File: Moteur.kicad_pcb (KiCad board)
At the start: 4 copper layers, 28 x 16 mm, 56 parts, among them IC1 TPS71501, IC2 TLV710, IC3 MAX3051, IC4 LM5106, IC5 LM5106, IC6 INA282, P1 Bus2, P2 MotorEnc, P3 Bus1, P4 Motor, P5 DBG, P6 PWR, P7 GPIO, Q1 IRF8721, Q2 IRF8721, Q3 IRF8721, Q4 IRF8721, U1 STM32F303CCT6, X1 16MHz

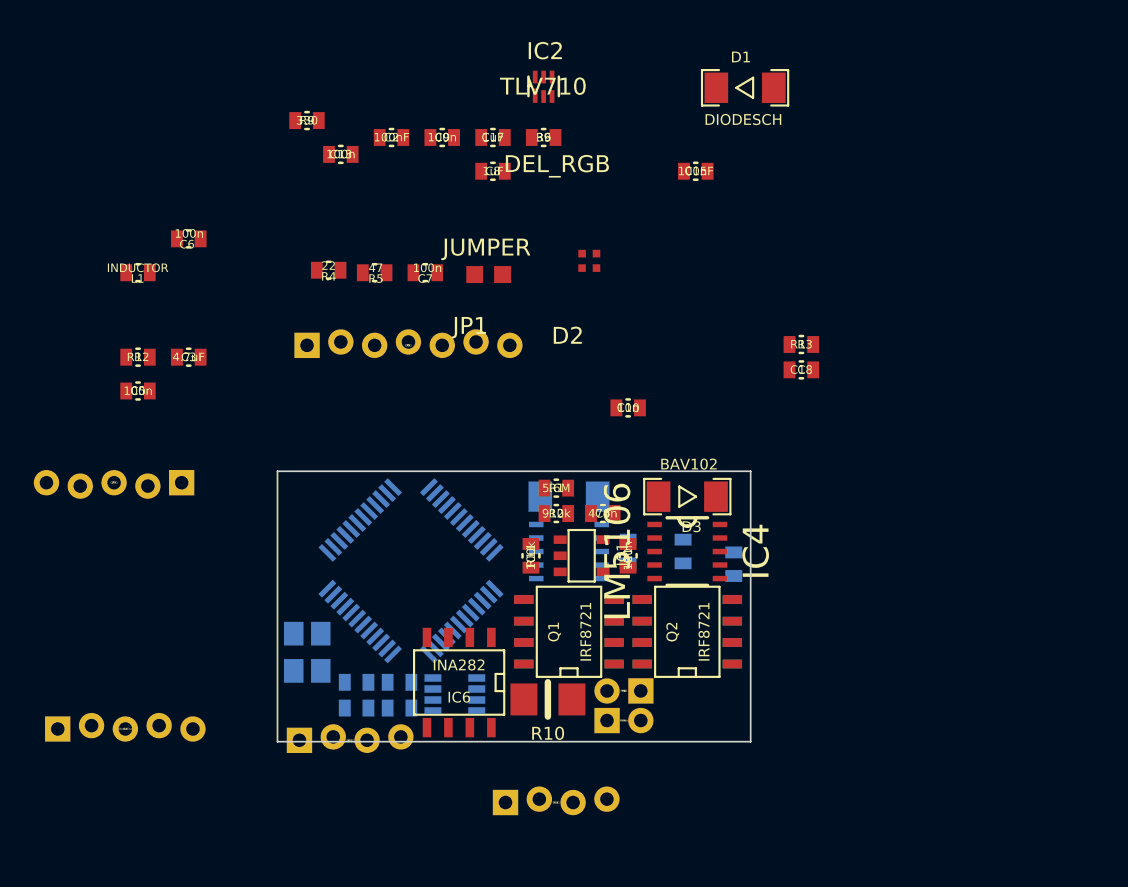
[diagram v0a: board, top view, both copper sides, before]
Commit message: final schematic review, component placement
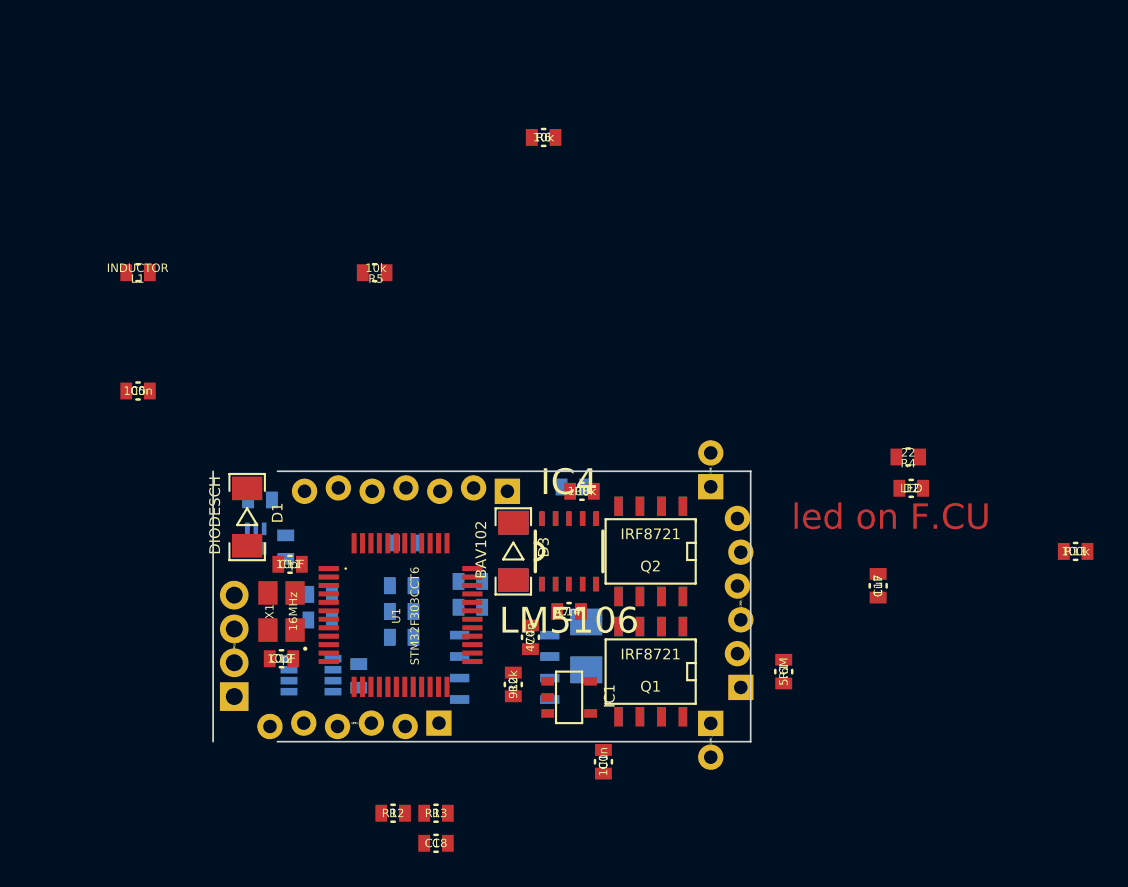
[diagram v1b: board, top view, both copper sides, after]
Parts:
- removed JP1: JUMPER, Jumer
- removed P7: GPIO, _Pin2mm_5z
- removed R7: 120, _0603
- C10, C13, C15, C2, C3, C6, C7, C8, C9, IC2, IC6, P5, R10, R9: moved to B.Cu
- C11, C12, C14, R8, U1, X1: moved to F.Cu
- D2: value DEL_RGB -> LED; footprint Led_RGB -> _0603
- P1: footprint _Pin2mm_4z -> pin4_can_connector
- P2: value MotorEnc -> CONN_6; footprint _Pin2mm_5z -> _Pin2mm_6z
- P3: value Bus1 -> GPIO; footprint _Pin2mm_4z -> _Pin2mm_6z
- P4: value Motor -> CONN_1
- P6: value PWR -> CONN_1
- R3: value 0R -> 10k
- R5: value 47 -> 10k
- R6: value 39 -> 10k
- moved D1 38.9 mm to (124.2, 92.7), turned to 270 degrees
- moved P2 37.2 mm to (153.4, 97.8), turned to 90 degrees
- moved R4 36.0 mm to (163.3, 89.2)
- moved C18 35.4 mm to (135.4, 112.0)
- moved R13 35.2 mm to (135.4, 110.2)
- moved C17 35.0 mm to (161.5, 96.8), turned to 270 degrees
- moved R11 32.2 mm to (173.2, 94.7), turned to 180 degrees
- moved IC2 31.7 mm to (124.7, 94.0)
- moved R12 30.9 mm to (132.8, 110.2)
- moved C13 30.9 mm to (130.8, 102.1), turned to 270 degrees
- moved R9 30.4 mm to (137.4, 98.0)
- moved C15 27.7 mm to (137.4, 96.5)
- moved C8 27.0 mm to (128.5, 97.3), turned to 180 degrees
- moved C9 26.6 mm to (133.3, 96.8)
- moved C6 25.4 mm to (133.3, 98.3)
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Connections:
- C15 pad 1: ADC/I_BAT -> ADC/I_MOT
- C5 pad 1: N-0000022 -> Reset
- IC3 pad 8: N-0000013 -> CAN_SPEED
- P2 pad 1: I -> Mot-
- P2 pad 2: B -> Mot+
- P2 pad 3: A -> GND
- P2 pad 4: GND -> +5V_protected
- P2 pad 5: +5V_protected -> B
- P3 pad 1: CANL -> GPIO_ADC
- P3 pad 2: CANH -> I
- P3 pad 3: GND -> GPIO_B
- P3 pad 4: +5V -> GPIO_A
- P4 pad 1: Mot- -> +BATT
- P4 pad 2: Mot+ -> (no net)
- P5 pad 3: (no net) -> Swdclk
- P5 pad 4: (no net) -> Swdio
- P5 pad 5: (no net) -> Reset
- P6 pad 2: +BATT -> (no net)
- R3 pad 1: N-0000012 -> +5V_protected
- R3 pad 2: N-0000013 -> GPIO_A
- R4 pad 1: N-0000068 -> LED
- R5 pad 1: N-0000069 -> +5V_protected
- R5 pad 2: N-0000067 -> GPIO_B
- R6 pad 1: LEDR -> +5V_protected
- R6 pad 2: N-0000046 -> I
- R9 pad 1: ADC/I_BAT -> ADC/I_MOT
- U1 pad 10: (no net) -> GPIO_ADC
- U1 pad 11: (no net) -> LED
- U1 pad 12: LEDR -> (no net)
- U1 pad 13: N-0000068 -> (no net)
- U1 pad 14: ADC/V_BAT -> CAN_SPEED
- U1 pad 15: (no net) -> ADC/I_MOT
- U1 pad 16: (no net) -> ADC/V_BAT
- U1 pad 19: I -> (no net)
- U1 pad 20: N-0000012 -> (no net)
- U1 pad 33: N-0000069 -> I
- U1 pad 34: (no net) -> Swdio
- U1 pad 37: (no net) -> Swdclk
- U1 pad 7: N-0000022 -> Reset
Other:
- board size 28 x 16 mm -> 31.8 x 16 mm
- board text added: "led on F.CU"
